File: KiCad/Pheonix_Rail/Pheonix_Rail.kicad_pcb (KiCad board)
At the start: 2 copper layers, 127 x 26 mm, 15 parts, among them J1 1729128, J10 1729128, J11 1729128, J12 1729128, J13 1729128, J2 1729128, J3 1729128, J4 1729128, J5 1729128, J6 1729128, J7 1729128, J8 1729128, J9 1729128

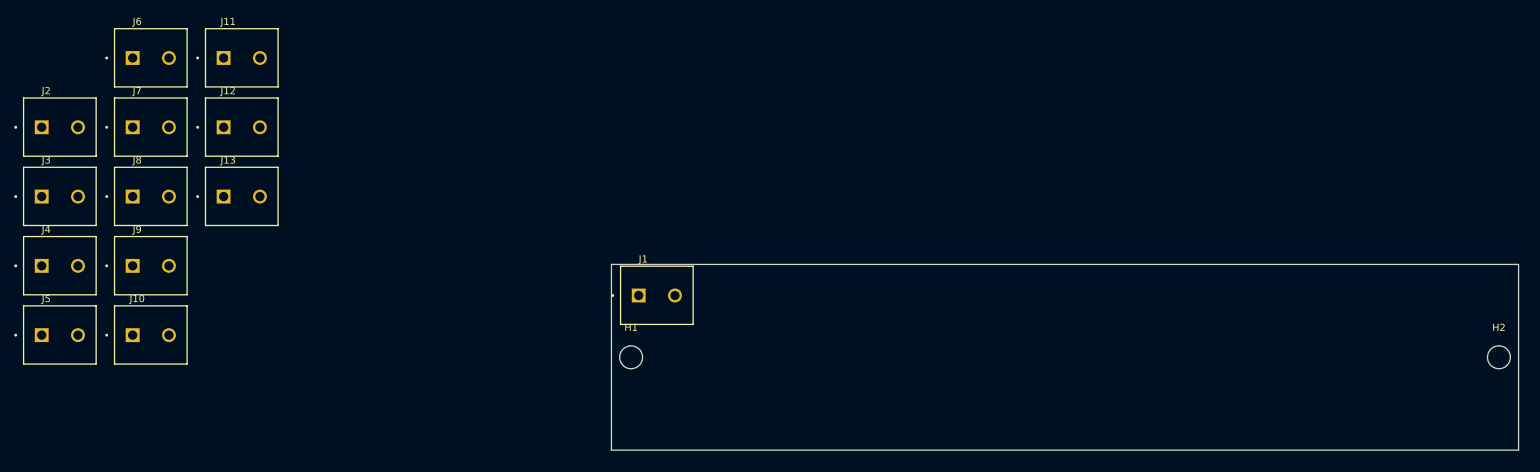
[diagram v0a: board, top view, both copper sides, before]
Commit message: layout for phoenix board
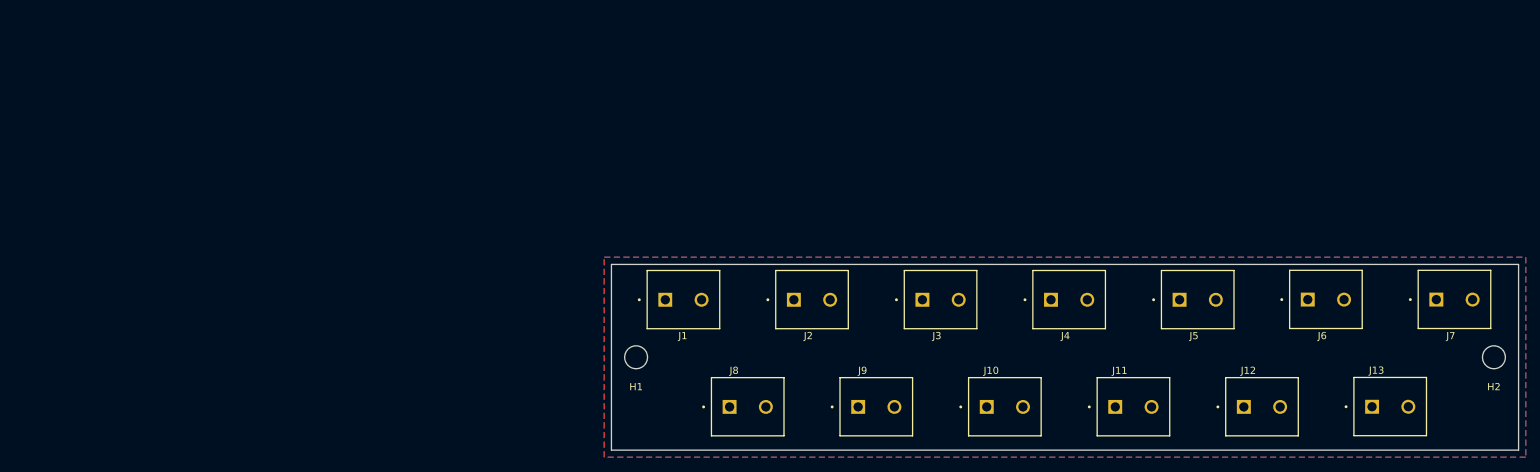
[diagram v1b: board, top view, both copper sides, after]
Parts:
- moved J7 184.1 mm to (255.9, 70.0)
- moved J6 168.0 mm to (237.9, 70.0)
- moved J13 163.5 mm to (246.9, 85.0)
- moved J5 159.4 mm to (220.0, 70.0)
- moved J12 148.1 mm to (229.0, 85.0)
- moved J4 141.4 mm to (202.0, 70.0)
- moved J11 134.1 mm to (211.0, 85.0)
- moved J3 124.1 mm to (184.0, 70.0)
- moved J10 120.0 mm to (193.0, 85.0)
- moved J2 108.0 mm to (166.0, 70.0)
- moved J9 103.5 mm to (175.0, 85.0)
- moved J8 88.6 mm to (157.0, 85.0)
- moved J1 3.77 mm to (148.0, 70.0)
- moved H1 0.70 mm to (146.4, 74.0), turned to 180 degrees
- moved H2 0.70 mm to (266.6, 74.0), turned to 180 degrees
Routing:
- added copper zone on F.Cu, net +24V
- added copper zone on B.Cu, net GND
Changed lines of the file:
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@@
 	(footprint "1729128:PHOENIX_1729128"
 		(layer "F.Cu")
-		(at 73.43 36.15)
+		(at 237.9475 69.975)
 		(property "Reference" "J6"
-			(at 3.175 -9.135 0)
+			(at 4.5675 1.025 0)
 			(layer "F.SilkS")
 			(effects
@@
 	(footprint "1729128:PHOENIX_1729128"
 		(layer "F.Cu")
-		(at 73.43 45.85)
+		(at 255.9475 69.975)
 		(property "Reference" "J7"
-			(at 3.175 -9.135 0)
+			(at 4.5675 1.025 0)
 			(layer "F.SilkS")
 			(effects
@@
 	(footprint "1729128:PHOENIX_1729128"
 		(layer "F.Cu")
-		(at 73.43 55.55)
+		(at 157 85)
 		(property "Reference" "J8"
 			(at 3.175 -9.135 0)
@@
 	(footprint "1729128:PHOENIX_1729128"
 		(layer "F.Cu")
-		(at 86.165 36.15)
+		(at 211 85)
 		(property "Reference" "J11"
 			(at 3.175 -9.135 0)
@@
 	(footprint "1729128:PHOENIX_1729128"
 		(layer "F.Cu")
-		(at 60.695 55.55)
+		(at 184 70)
 		(property "Reference" "J3"
-			(at 3.175 -9.135 0)
+			(at 4.5675 1 0)
 			(layer "F.SilkS")
 			(effects
@@
 	(footprint "1729128:PHOENIX_1729128"
 		(layer "F.Cu")
-		(at 86.165 55.55)
+		(at 246.9475 84.975)
 		(property "Reference" "J13"
 			(at 3.175 -9.135 0)
@@
 	(footprint "1729128:PHOENIX_1729128"
 		(layer "F.Cu")
-		(at 86.165 45.85)
+		(at 229 85)
 		(property "Reference" "J12"
 			(at 3.175 -9.135 0)
@@
 	(footprint "MountingHole:MountingHole_3.2mm_M3"
 		(layer "F.Cu")
-		(at 145.75 74)
+		(at 146.45 74 180)
 		(descr "Mounting Hole 3.2mm, M3, no annular, generated by kicad-footprint-generator mountinghole.py")
 		(tags "mountinghole M3")
@@
 		)
 		(pad "" np_thru_hole circle
-			(at 0 0)
+			(at 0 0 180)
 			(size 3.2 3.2)
 			(drill 3.2)
@@
 	(footprint "1729128:PHOENIX_1729128"
 		(layer "F.Cu")
-		(at 60.695 74.95)
+		(at 220 70)
 		(property "Reference" "J5"
-			(at 3.175 -9.135 0)
+			(at 4.5675 1 0)
 			(layer "F.SilkS")
 			(effects
@@
 	(footprint "1729128:PHOENIX_1729128"
 		(layer "F.Cu")
-		(at 73.43 65.25)
+		(at 175 85)
 		(property "Reference" "J9"
 			(at 3.175 -9.135 0)
@@
 	(footprint "1729128:PHOENIX_1729128"
 		(layer "F.Cu")
-		(at 73.43 74.95)
+		(at 193 85)
 		(property "Reference" "J10"
 			(at 3.175 -9.135 0)
@@
 	(footprint "1729128:PHOENIX_1729128"
 		(layer "F.Cu")
-		(at 144.275 69.4)
+		(at 148 70)
 		(property "Reference" "J1"
-			(at 3.175 -9.135 0)
+			(at 5 1 0)
 			(layer "F.SilkS")
 			(effects
@@
 	(footprint "1729128:PHOENIX_1729128"
 		(layer "F.Cu")
-		(at 60.695 65.25)
+		(at 202 70)
 		(property "Reference" "J4"
-			(at 3.175 -9.135 0)
+			(at 4.5675 1 0)
 			(layer "F.SilkS")
 			(effects
@@
 	(footprint "1729128:PHOENIX_1729128"
 		(layer "F.Cu")
-		(at 60.695 45.85)
+		(at 166 70)
 		(property "Reference" "J2"
-			(at 3.175 -9.135 0)
+			(at 4.5675 1 0)
 			(layer "F.SilkS")
 			(effects
@@
 	(footprint "MountingHole:MountingHole_3.2mm_M3"
 		(layer "F.Cu")
-		(at 267.25 74)
+		(at 266.55 74 180)
 		(descr "Mounting Hole 3.2mm, M3, no annular, generated by kicad-footprint-generator mountinghole.py")
 		(tags "mountinghole M3")
@@
 		)
 		(pad "" np_thru_hole circle
-			(at 0 0)
+			(at 0 0 180)
 			(size 3.2 3.2)
 			(drill 3.2)
@@
 		)
 		(fill no)
+		(locked yes)
 		(layer "Edge.Cuts")
 	)
+	(zone
+		(net 1)
+		(net_name "+24V")
+		(layer "F.Cu")
+		(hatch edge 0.5)
+		(connect_pads
+			(clearance 0.5)
+		)
+		(min_thickness 0.25)
+		(filled_areas_thickness no)
+		(fill yes
+			(thermal_gap 0.5)
+			(thermal_bridge_width 0.5)
+		)
+		(polygon
+			(pts
+				(xy 142 60) (xy 271 60) (xy 271 88) (xy 142 88)
+			)
+		)
+	)
+	(zone
+		(net 2)
+		(net_name "GND")
+		(layer "B.Cu")
+		(hatch edge 0.5)
+		(priority 1)
+		(connect_pads
+			(clearance 0.5)
+		)
+		(min_thickness 0.25)
+		(filled_areas_thickness no)
+		(fill yes
+			(thermal_gap 0.5)
+			(thermal_bridge_width 0.5)
+		)
+		(polygon
+			(pts
+				(xy 142 60) (xy 271 60) (xy 271 88) (xy 142 88)
+			)
+		)
+	)
 	(embedded_fonts no)
